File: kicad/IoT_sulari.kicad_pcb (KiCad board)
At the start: 4 copper layers, 50.7 x 41 mm, 45 parts, among them J1 73412-0110, J2 73412-0110, J20 694106106102, J3 20021121-00010C4LF, J4 20021121-00010C4LF, J40 693043020611, J5 10129380-908001ALF, SW1 SW_SPST, SW2 TL3301DF160QG, SW3 TL3301DF160QG, SW4 TL3301DF160QG, SW5 TL3301DF160QG, U2 NRF9160, U20 MIC5219-3.3YM5-TR, U40 TPD3F303DPVR

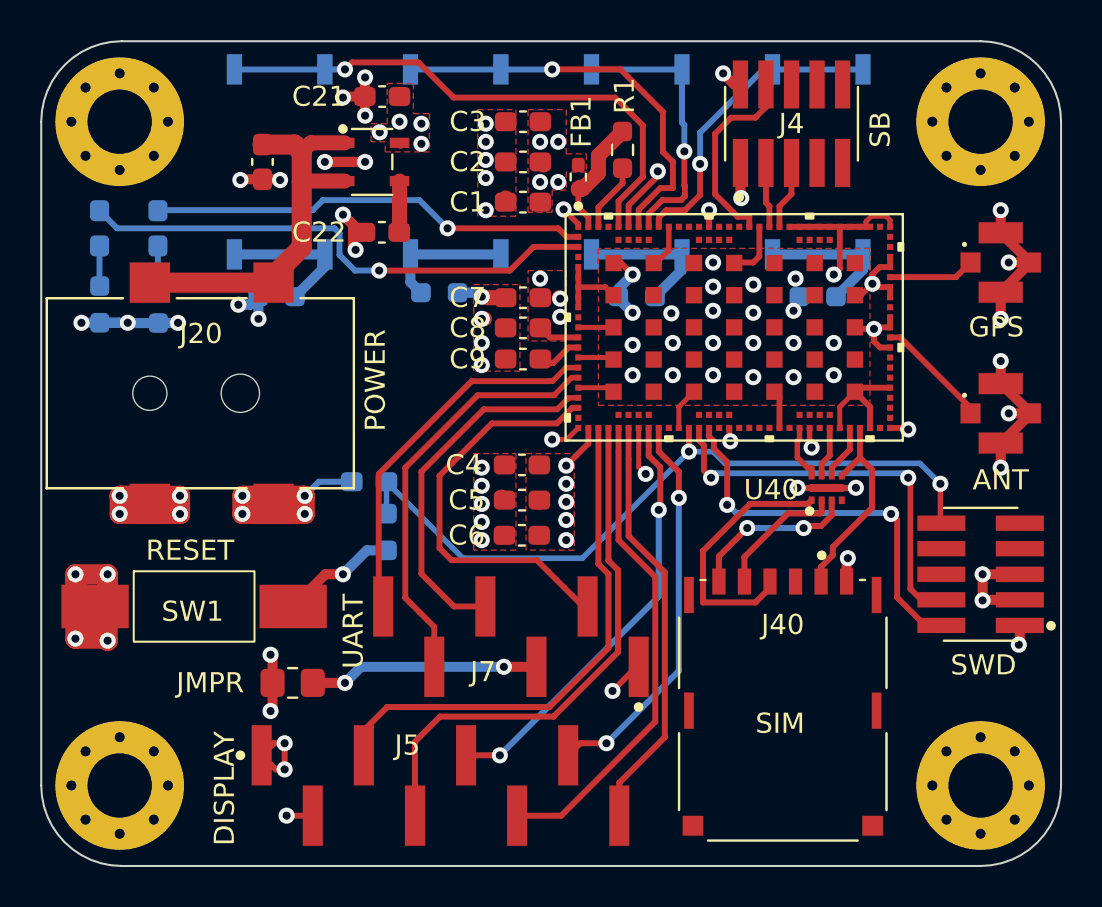
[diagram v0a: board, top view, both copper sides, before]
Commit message: ESD change
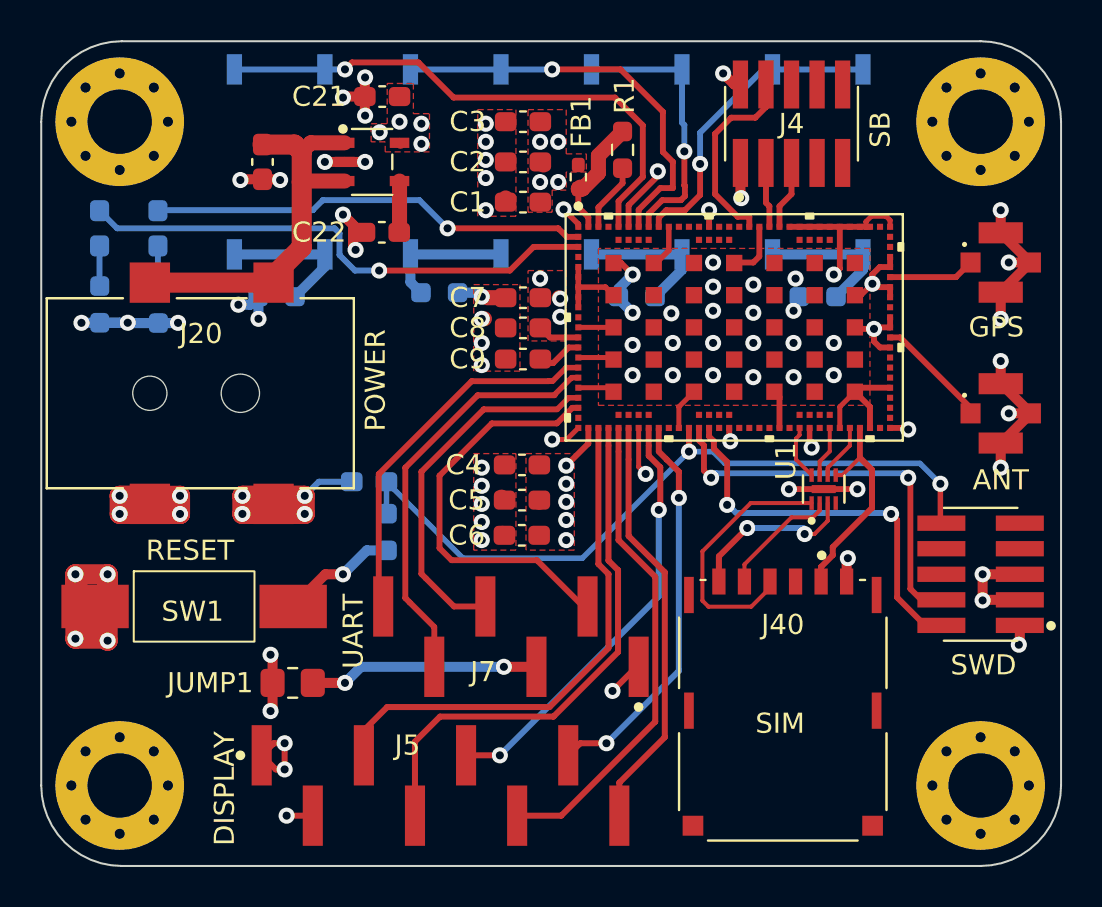
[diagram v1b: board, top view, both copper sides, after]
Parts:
- removed U40: TPD3F303DPVR, TPD3F303DPVR:TPD3F303DPVR
- added U1: TPD3F303DQDR, TPD3F303DQDR:TPD3F303DQDR, F.Cu at (131.2, 57.3)
- renumbered JMPR to JUMP1
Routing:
- net GND: track 156.9 -> 157.4 mm

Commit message: Revert "ESD change"
This reverts commit acabe66db7bce87ed7ccd6d28b87d0a8866a87e9.
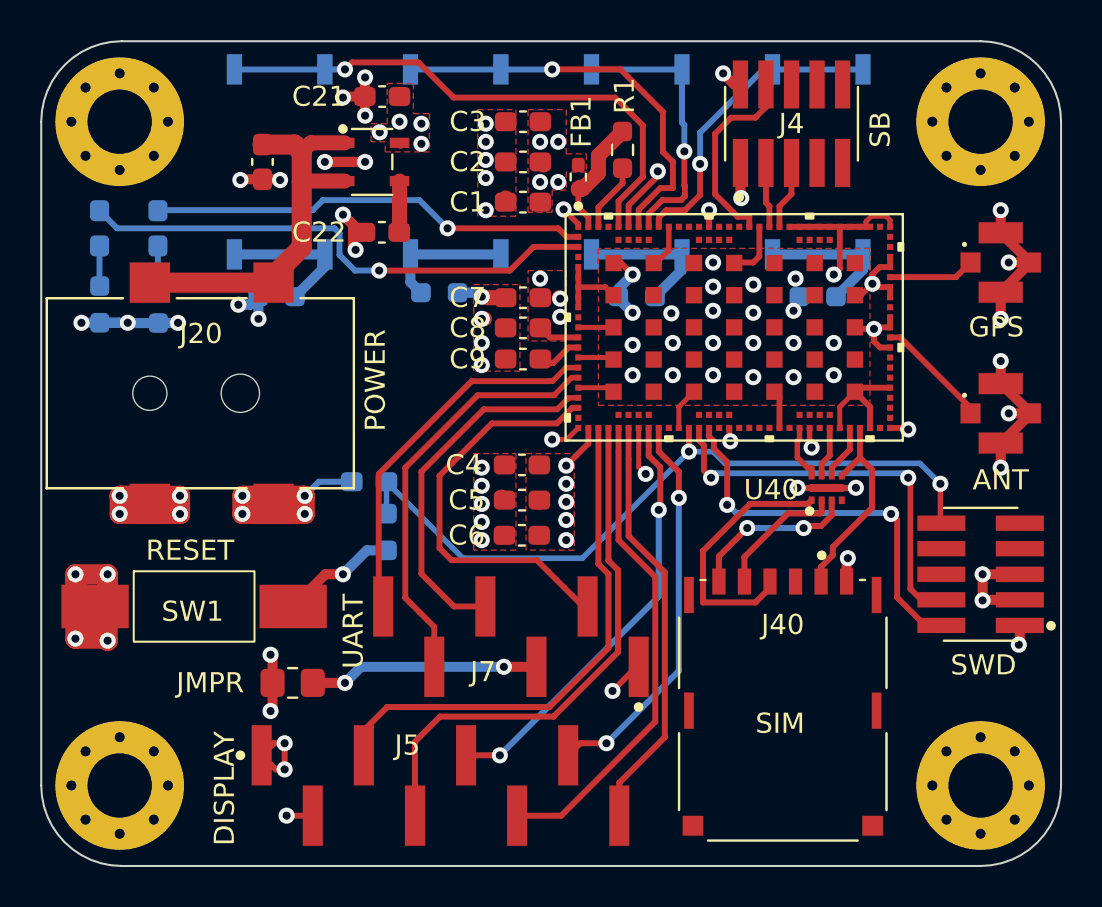
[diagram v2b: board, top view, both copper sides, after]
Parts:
- removed U1: TPD3F303DQDR, TPD3F303DQDR:TPD3F303DQDR
- added U40: TPD3F303DPVR, TPD3F303DPVR:TPD3F303DPVR, F.Cu at (131.4, 57.2)
- renumbered JUMP1 to JMPR
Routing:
- net GND: track 157.4 -> 156.9 mm
